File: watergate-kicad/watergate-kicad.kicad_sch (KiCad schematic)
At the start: 16 parts, among them IC1 DHT22, U1 ESP32-DEVKITC-32D

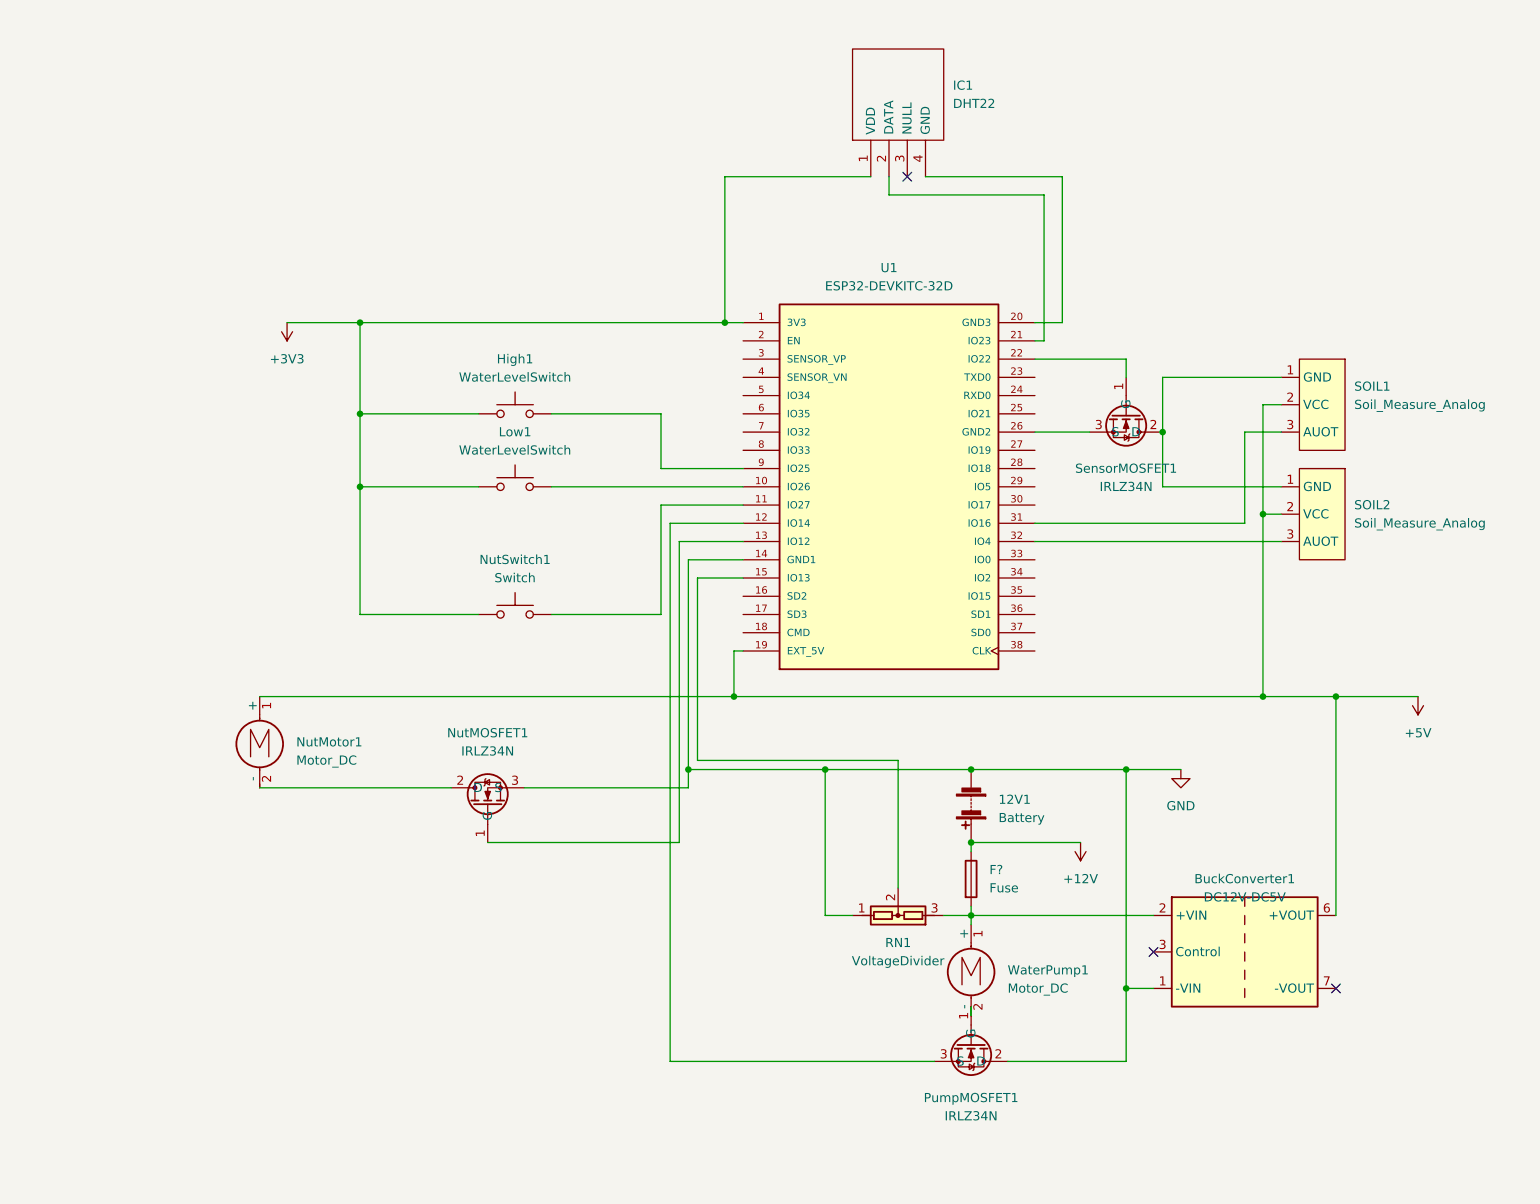
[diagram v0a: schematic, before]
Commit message: Update to reality
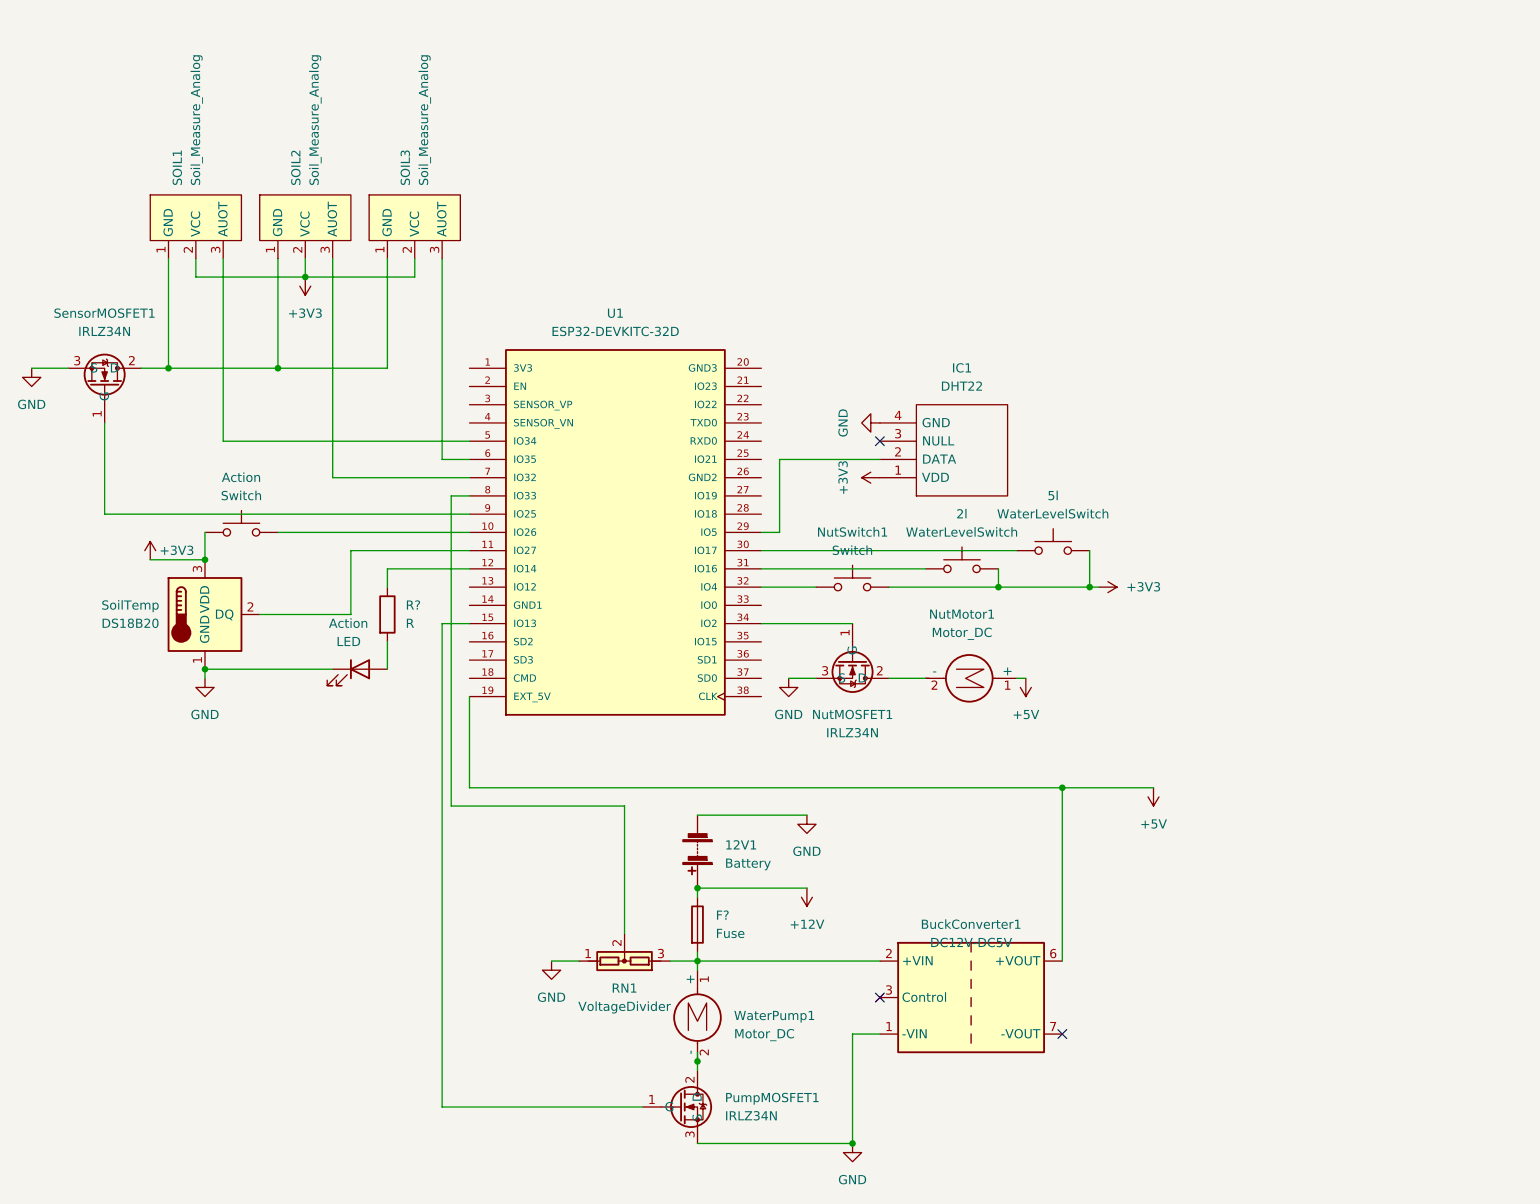
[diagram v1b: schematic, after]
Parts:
- added Action: Switch, Package_DIP:DIP-8_W7.62mm, symbol Switch:SW_Push
- added Action: LED, symbol Device:LED
- added R?: R, symbol Device:R
- added SOIL3: Soil_Measure_Analog, Connector_JST:JST_VH_B3P-VH-FB-B_1x03_P3.96mm_Vertical, symbol Gotling:Soil_Measure_Analog
- added SoilTemp: DS18B20, Package_TO_SOT_THT:TO-92_Inline, symbol Sensor_Temperature:DS18B20
- renumbered Low1 to 2l, High1 to 5l
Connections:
- net +3V3: now also 2l.2, 5l.2, NutSwitch1.2, SOIL1.2 (VCC), SOIL2.2 (VCC), Action.1, SOIL3.2 (VCC), SoilTemp.3 (VDD); no longer 2l.1, 5l.1, NutSwitch1.1, U1.1 (3V3)
- net +5V: no longer SOIL1.2 (VCC), SOIL2.2 (VCC)
- net GND: now also IC1.4 (GND), PumpMOSFET1.3 (S), SensorMOSFET1.3 (S), Action.1 (K), SoilTemp.1 (GND); no longer PumpMOSFET1.2 (D), U1.14 (GND1)
- net at SOIL1.1 (GND), SOIL2.1 (GND), SensorMOSFET1.2 (D): now also SOIL3.1 (GND)
- net at SOIL1.3 (AUOT): now also U1.5 (IO34); no longer U1.31 (IO16)
- net at PumpMOSFET1.1 (G): now also U1.15 (IO13); no longer WaterPump1.2 (-)
- net at U1.12 (IO14): now also R?.1; no longer PumpMOSFET1.3 (S)
- net at U1.10 (IO26): now also Action.2; no longer 2l.2
- net at U1.9 (IO25): now also SensorMOSFET1.1 (G); no longer 5l.2
- net at SOIL2.3 (AUOT): now also U1.7 (IO32); no longer U1.32 (IO4)
- net at U1.11 (IO27): now also SoilTemp.2 (DQ); no longer NutSwitch1.2
- net at U1.13 (IO12): no longer NutMOSFET1.1 (G)
- net at RN1.2: now also U1.8 (IO33); no longer U1.15 (IO13)
- net at U1.20 (GND3): no longer IC1.4 (GND)
- net at U1.21 (IO23): no longer IC1.2 (DATA)
- net at U1.22 (IO22): no longer SensorMOSFET1.1 (G)
- net at U1.26 (GND2): no longer SensorMOSFET1.3 (S)
- net at U1.29 (IO5): now also IC1.2 (DATA)
- net at U1.30 (IO17): now also 5l.1
- net at U1.34 (IO2): now also NutMOSFET1.1 (G)
- net at U1.6 (IO35): now also SOIL3.3 (AUOT)
- new net: PumpMOSFET1.2 (D), WaterPump1.2 (-)
- new net: 2l.1, U1.31 (IO16)
- new net: NutSwitch1.1, U1.32 (IO4)
- new net: Action.2 (A), R?.2
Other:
- moved on the sheet: 12V1, 2l, 5l, BuckConverter1, F?, IC1, NutMOSFET1, NutMotor1, NutSwitch1, PumpMOSFET1, RN1, SOIL1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
